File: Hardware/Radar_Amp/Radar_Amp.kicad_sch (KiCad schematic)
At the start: 38 parts, among them J1 Conn_Supply, J2 Conn_Radar, U2 OPA_REF, U4 OPA_DRIVER, U9 TPS7A20

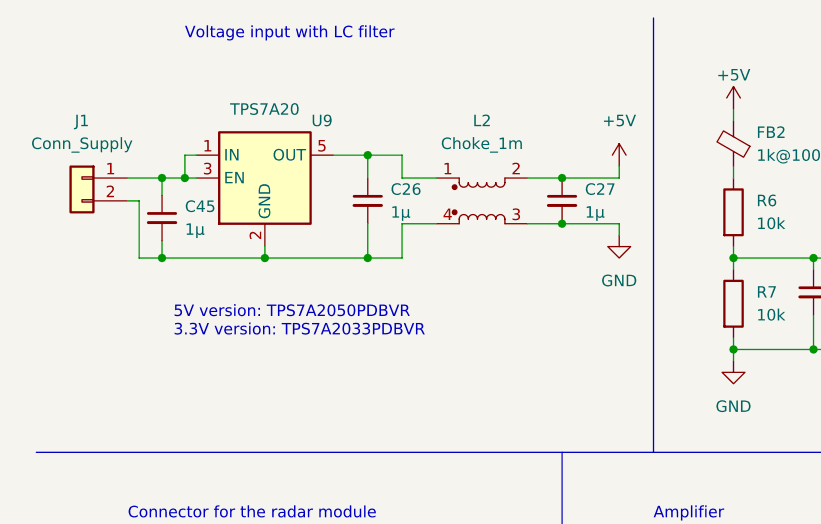
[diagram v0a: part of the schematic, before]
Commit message: update
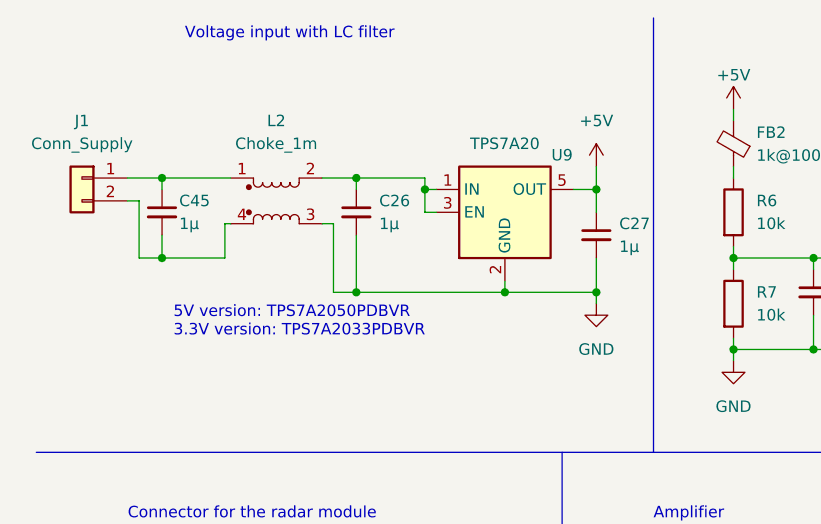
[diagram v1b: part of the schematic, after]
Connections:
- net +5V: now also U9.5 (OUT); no longer L2.2
- net GND: now also C26.2, U9.2 (GND)
- net at C45.2, J1.2 (Pin_2), L2.4: no longer C26.2, U9.2 (GND)
- net at U9.1 (IN), U9.3 (EN): now also C26.1, L2.2; no longer C45.1, J1.1 (Pin_1)
- new net: C45.1, J1.1 (Pin_1), L2.1
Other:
- moved on the sheet: C26, C27, C45, L2, U9
